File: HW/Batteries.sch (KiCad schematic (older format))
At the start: 18 parts, among them J2 Batt1, J3 Batt1, J4 Batt1, Q4 FS8205, Q5 FS8205, Q6 FS8205, U15 DW01-P, U16 DW01-P, U17 DW01-P

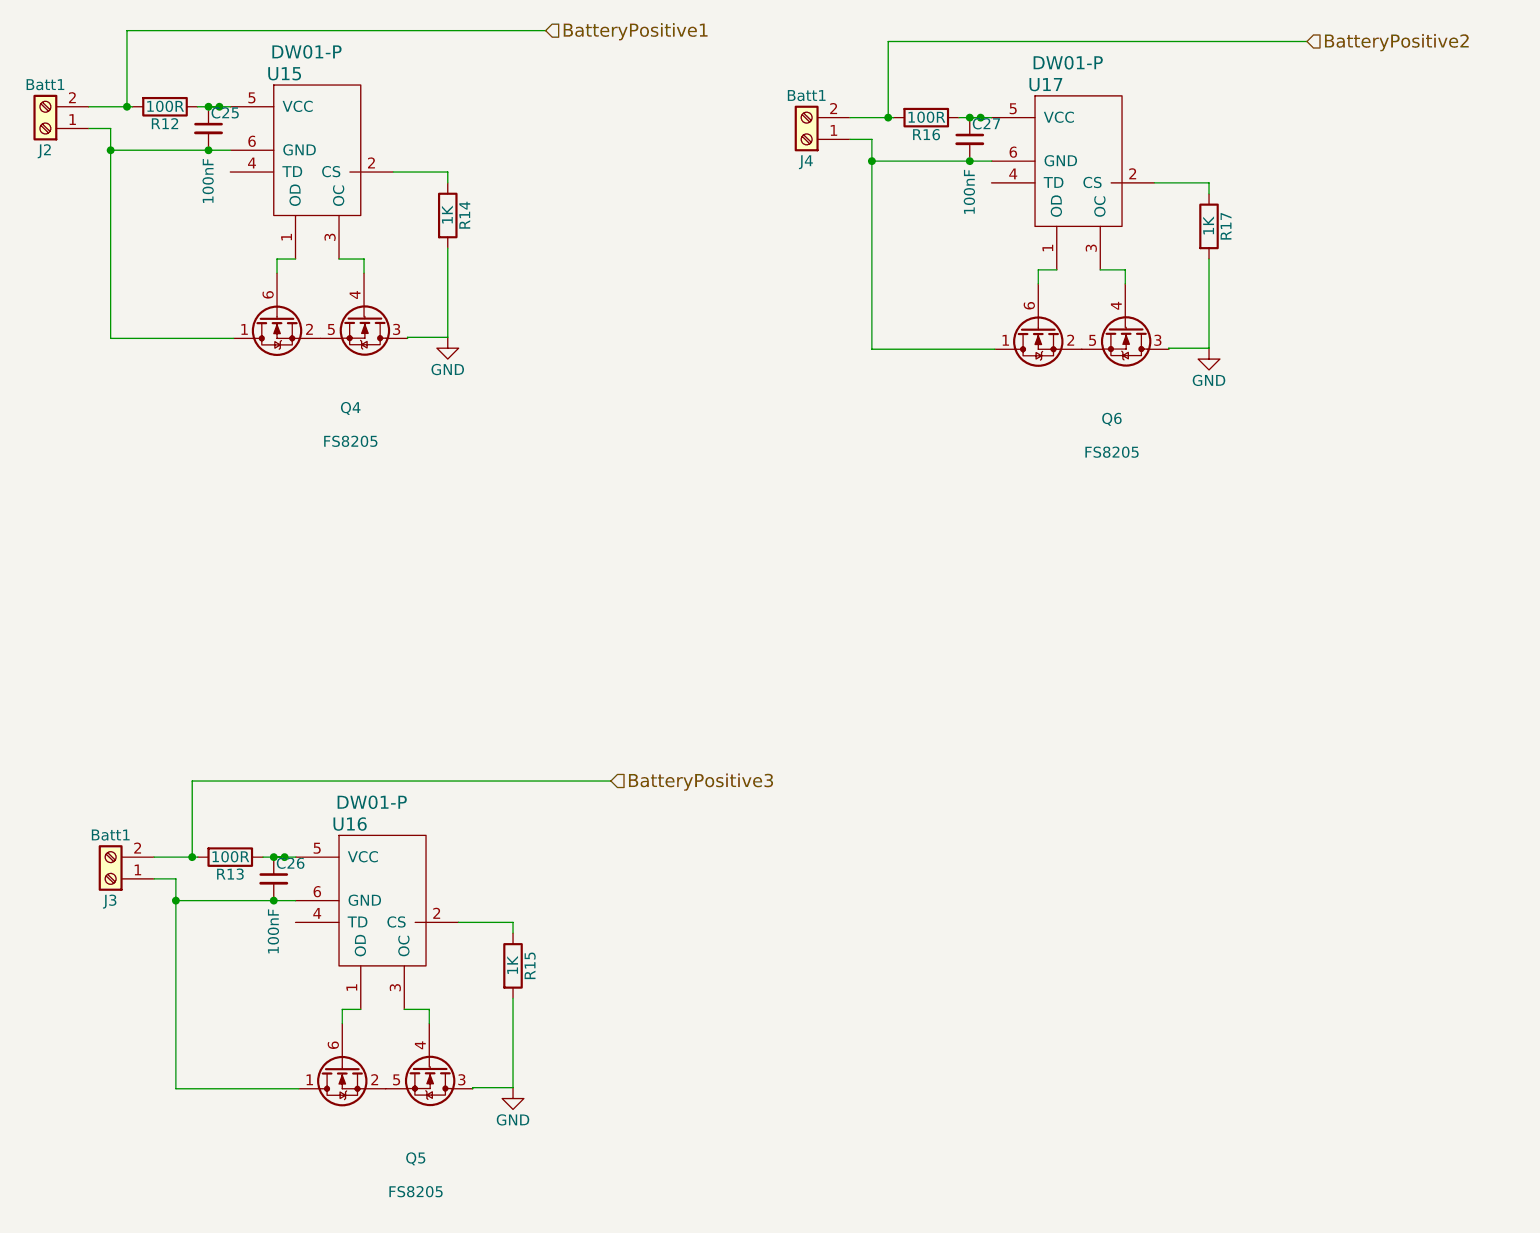
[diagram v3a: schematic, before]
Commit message: Add files via upload
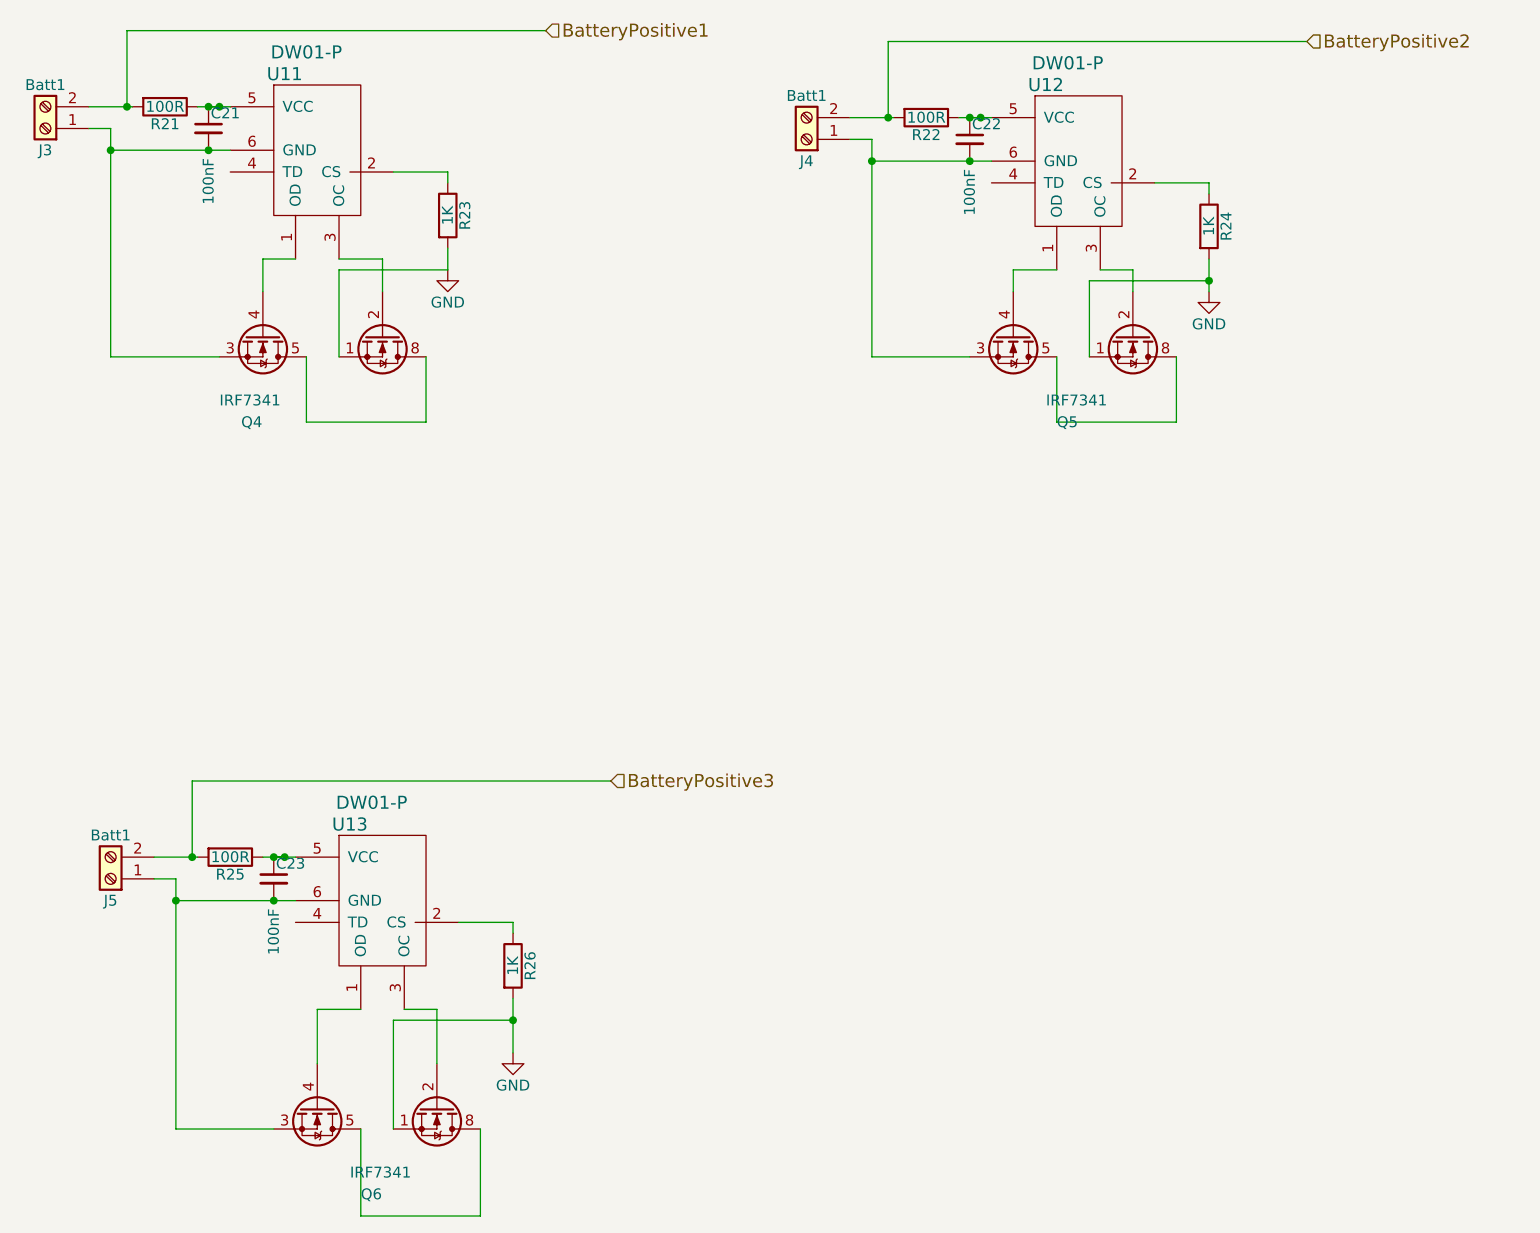
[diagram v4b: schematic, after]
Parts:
- removed Q4, Q5, Q6: FS8205, TO_SOT_Packages_SMD:SOT-23-6_Handsoldering, symbol FS8205
- added Q4, Q5, Q6: IRF7341, Housings_SOIC:SO-8_5.3x6.2mm_Pitch1.27mm, symbol IRF7341
- renumbered C25 to C21, C27 to C22, C26 to C23, J2 to J3, J3 to J5, R12 to R21, R16 to R22, R14 to R23, R17 to R24, R13 to R25, R15 to R26, U15 to U11, U17 to U12, U16 to U13
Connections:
- net GND: now also Q4.1 (S1), Q5.1 (S1), Q6.1 (S1)
- net at C22.2, J4.1 (Pin_1), U12.6 (GND): now also Q5.3 (S2)
- net at U12.3 (OC): now also Q5.2 (G1)
- net at U12.1 (OD): now also Q5.4 (G2)
- net at C21.2, J3.1 (Pin_1), U11.6 (GND): now also Q4.3 (S2)
- net at U11.3 (OC): now also Q4.2 (G1)
- net at U11.1 (OD): now also Q4.4 (G2)
- net at C23.2, J5.1 (Pin_1), U13.6 (GND): now also Q6.3 (S2)
- net at U13.3 (OC): now also Q6.2 (G1)
- net at U13.1 (OD): now also Q6.4 (G2)
- new net: Q4.5 (D2), Q4.8 (D1)
- new net: Q5.5 (D2), Q5.8 (D1)
- new net: Q6.5 (D2), Q6.8 (D1)

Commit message: Add files via upload
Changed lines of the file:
@@
 $EndComp
 Wire Wire Line
-	5500 1600 5550 1600
-Wire Wire Line
-	5550 1600 5600 1600
-Wire Wire Line
-	5600 1600 5650 1600
+	5500 1600 5650 1600
 Wire Wire Line
 	6400 1900 6650 1900
@@
 	6650 1900 6650 1950
 Wire Wire Line
-	5000 1600 5175 1600
-Wire Wire Line
-	5175 1600 5200 1600
+	5000 1600 5200 1600
 Wire Wire Line
 	5175 1600 5175 1250
@@
 	5100 1700 5000 1700
 Wire Wire Line
-	5100 1800 5550 1800
-Wire Wire Line
-	5550 1800 5650 1800
+	5100 1800 5650 1800
 $Comp
 L R R21
@@
 $EndComp
 Wire Wire Line
-	2000 1550 2050 1550
-Wire Wire Line
-	2050 1550 2100 1550
-Wire Wire Line
-	2100 1550 2150 1550
+	2000 1550 2150 1550
 Wire Wire Line
 	2900 1850 3150 1850
@@
 	3150 1850 3150 1900
 Wire Wire Line
-	1500 1550 1675 1550
-Wire Wire Line
-	1675 1550 1700 1550
+	1500 1550 1700 1550
 Wire Wire Line
 	1675 1550 1675 1200
@@
 $EndComp
 Wire Wire Line
-	2300 5000 2350 5000
-Wire Wire Line
-	2350 5000 2400 5000
-Wire Wire Line
-	2400 5000 2450 5000
+	2300 5000 2450 5000
 Wire Wire Line
 	3200 5300 3450 5300
@@
 	3450 5300 3450 5350
 Wire Wire Line
-	1800 5000 1975 5000
-Wire Wire Line
-	1975 5000 2000 5000
+	1800 5000 2000 5000
 Wire Wire Line
 	1975 5000 1975 4650
@@
 	1900 5100 1800 5100
 Wire Wire Line
-	1900 5200 2350 5200
-Wire Wire Line
-	2350 5200 2450 5200
+	1900 5200 2450 5200
 $Comp
 L IRF7341 Q4
@@
 	1600 2700 2100 2700
 Wire Wire Line
-	1600 1650 1600 1750
-Wire Wire Line
-	1600 1750 1600 2700
-Wire Wire Line
-	1600 1750 2050 1750
-Wire Wire Line
-	2050 1750 2150 1750
+	1600 1650 1600 2700
+Wire Wire Line
+	1600 1750 2150 1750
 Connection ~ 1600 1750
 $Comp
@@
 	5100 2700 5550 2700
 Wire Wire Line
-	5100 1700 5100 1800
-Wire Wire Line
-	5100 1800 5100 2700
+	5100 1700 5100 2700
 Wire Wire Line
 	6100 2350 6100 2700
@@
 	6100 2350 6650 2350
 Wire Wire Line
-	6650 2250 6650 2350
-Wire Wire Line
-	6650 2350 6650 2400
+	6650 2250 6650 2400
 $Comp
 L GND #PWR067
@@
 	2900 5750 3450 5750
 Wire Wire Line
-	3450 5650 3450 5750
-Wire Wire Line
-	3450 5750 3450 5900
+	3450 5650 3450 5900
 Connection ~ 3450 5750
 Wire Wire Line
@@
 	1900 6250 2350 6250
 Wire Wire Line
-	1900 5100 1900 5200
-Wire Wire Line
-	1900 5200 1900 6250
+	1900 5100 1900 6250
 $Comp
 L GND #PWR068
